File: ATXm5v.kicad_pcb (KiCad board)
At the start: 4 copper layers, 80 x 47 mm, 41 parts, among them J1 Power Switch, J2 ATX, J3 AT, J4 Power LED, SW1 Power, U1 74HC74, U2 74HC14, U3 L7905, U4 74HC4060, U5 74HC73, Y1 3.2768

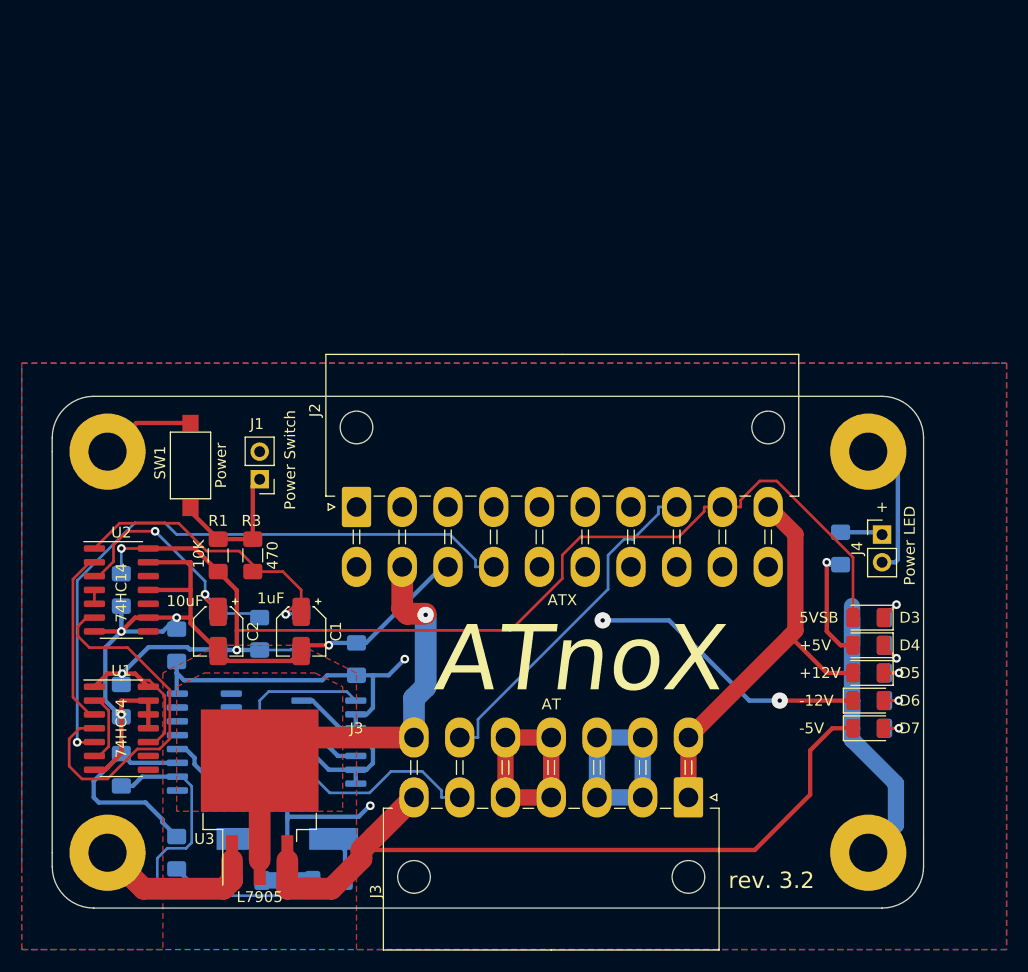
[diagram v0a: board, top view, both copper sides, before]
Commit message: Add initial pcb
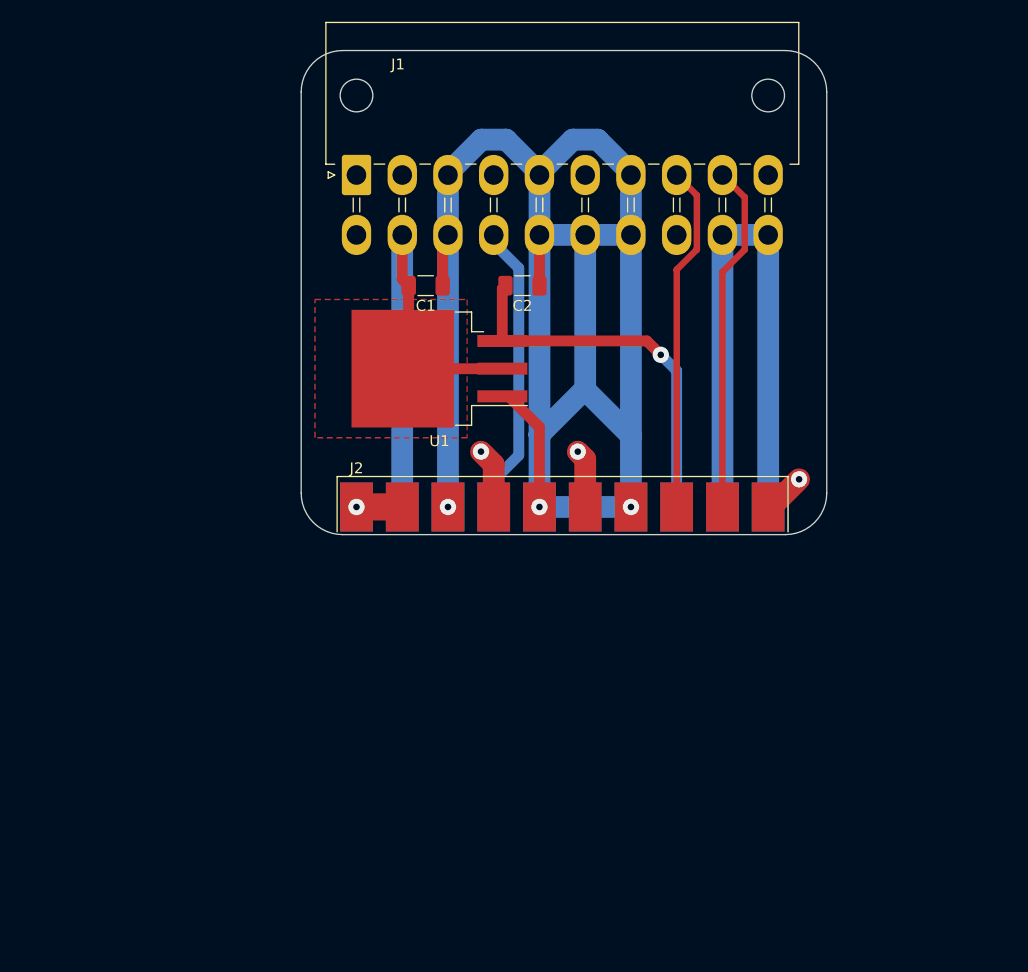
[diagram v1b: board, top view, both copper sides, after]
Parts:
- removed C3, C4, C5, C6: 100nF, Capacitor_SMD:C_1206_3216Metric_Pad1.42x1.75mm_HandSolder
- removed C7, C8: 6.8pF, Capacitor_SMD:C_1206_3216Metric_Pad1.42x1.75mm_HandSolder
- removed D1, D2: LL4148, Diode_SMD:D_MiniMELF
- removed D3: 5VSB, LED_SMD:LED_1206_3216Metric
- removed D4: +5V, LED_SMD:LED_1206_3216Metric
- removed D5: +12V, LED_SMD:LED_1206_3216Metric
- removed D6: -12V, LED_SMD:LED_1206_3216Metric
- removed D7: -5V, LED_SMD:LED_1206_3216Metric
- removed H1, H2, H3, H4: MountingHole_Pad, MountingHole:MountingHole_3.5mm_Pad
- removed J3: AT, Connector_Molex:Molex_Mini-Fit_Jr_5569-14A2_2x07_P4.20mm_Horizontal
- removed J4: Power LED, Connector_PinHeader_2.54mm:PinHeader_1x02_P2.54mm_Vertical
- removed R1, R2: 10K, Resistor_SMD:R_1206_3216Metric_Pad1.42x1.75mm_HandSolder
- removed R10: 100K, Resistor_SMD:R_1206_3216Metric_Pad1.42x1.75mm_HandSolder
- removed R11: 10M, Resistor_SMD:R_1206_3216Metric_Pad1.42x1.75mm_HandSolder
- removed R3, R5: 470, Resistor_SMD:R_1206_3216Metric_Pad1.42x1.75mm_HandSolder
- removed R4, R8: 680, Resistor_SMD:R_1206_3216Metric_Pad1.42x1.75mm_HandSolder
- removed R6, R7: 2k2, Resistor_SMD:R_1206_3216Metric_Pad1.42x1.75mm_HandSolder
- removed R9: 1K, Resistor_SMD:R_1206_3216Metric_Pad1.42x1.75mm_HandSolder
- removed SW1: Power, Button_Switch_SMD:SW_SPST_CK_RS282G05A3
- removed U2: 74HC14, Package_SO:SOIC-14_3.9x8.7mm_P1.27mm
- removed U3: L7905, Package_TO_SOT_SMD:TO-263-3_TabPin2
- removed U4: 74HC4060, Package_SO:SOIC-16_3.9x9.9mm_P1.27mm
- removed U5: 74HC73, Package_SO:SOIC-14_3.9x8.7mm_P1.27mm
- removed Y1: 3.2768, Crystal:Crystal_SMD_HC49-SD
- C1: value 1uF -> 10uF; footprint Capacitor_SMD:CP_Elec_4x5.3 -> Capacitor_SMD:C_1206_3216Metric_Pad1.33x1.80mm_HandSolder
- C2: value 10uF -> 100nF; footprint Capacitor_SMD:CP_Elec_4x5.3 -> Capacitor_SMD:C_1206_3216Metric_Pad1.33x1.80mm_HandSolder
- J1: value Power Switch -> ATX IN; footprint Connector_PinHeader_2.54mm:PinHeader_1x02_P2.54mm_Vertical -> Connector_Molex:Molex_Mini-Fit_Jr_5569-20A2_2x10_P4.20mm_Horizontal
- J2: value ATX -> ATX OUT; footprint Connector_Molex:Molex_Mini-Fit_Jr_5569-20A2_2x10_P4.20mm_Horizontal -> ATXm5v:ATX-Edge
- U1: value 74HC74 -> L7905; footprint Package_SO:SOIC-14_3.9x8.7mm_P1.27mm -> Package_TO_SOT_SMD:TO-263-3_TabPin2
- moved U1 44.1 mm to (135.9, 64.8), turned to 180 degrees
- moved C2 42.3 mm to (143.5, 57.1), turned to 180 degrees
- moved C1 33.7 mm to (134.6, 57.1), turned to 180 degrees
- moved J1 29.3 mm to (128.3, 47.0), turned to 0 degrees
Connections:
- C1 pad 1: Net-(C1-Pad1) -> GND
- C1 pad 2: GND -> /-12V
- C2 pad 1: Net-(C2-Pad1) -> GND
- C2 pad 2: GND -> /-5V
- J1 pad 1: /PWR_SW -> /3.3V
- J1 pad 2: GND -> /3.3V
- J2 pad 1: (no net) -> /3.3V
- J2 pad 11: (no net) -> /3.3V
- J2 pad 18: (no net) -> /-5V
- J2 pad 2: (no net) -> /3.3V
- U1 pad 1: /5VSB -> GND
- U1 pad 2: Net-(U1-Pad2) -> /-12V
- U1 pad 3: Net-(U1-Pad3) -> /-5V
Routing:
- net GND: track 415.8 -> 178.2 mm, vias 5 -> 3
- net /5VSB: track 125.1 -> 32.2 mm, vias 3 -> 0
- net /-12V: track 89.8 -> 46.9 mm, vias 3 -> 0
- net Net-(C8-Pad1): track 41.2 -> 0.00 mm
- net /3.3V: track 0.00 -> 38.9 mm, vias 0 -> 1
- net /-5V: track 71.0 -> 34.8 mm, vias 0 -> 1
- net VCC: track 210.2 -> 175.1 mm
- net Net-(U1-Pad4): track 34.2 -> 0.00 mm
- net /~PS_ON: track 58.9 -> 26.9 mm, vias 1 -> 0
- net Net-(C1-Pad1): track 28.5 -> 0.00 mm, vias 1 -> 0
- net Net-(C2-Pad1): track 24.3 -> 0.00 mm, vias 2 -> 0
- net Net-(R10-Pad1): track 20.4 -> 0.00 mm
- net /TICK: track 17.5 -> 0.00 mm
- net Net-(U1-Pad3): track 16.1 -> 0.00 mm
- net Net-(U4-Pad3): track 14.4 -> 0.00 mm
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- removed copper zone on B.Cu, net GND
- removed copper zone on F.Cu, net GND
- removed copper zone on In2.Cu, net GND
- removed copper zone on In1.Cu, net VCC
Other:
- board size 80 x 47 mm -> 48.3 x 44.5 mm
- board text removed: "+"
- board text removed: "+12V"
- board text removed: "+5V"
- board text removed: "-12V"
- board text removed: "-5V"
- board text removed: "5VSB"
- board text removed: "ATX Power Connector"
- board text removed: "ATnoX"
- board text removed: "Design by"
- board text removed: "Power Adapter Cable"
- board text removed: "rev. 3.2"
- board text removed: "tabaglio@posteo.net"
